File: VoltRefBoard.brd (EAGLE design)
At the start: 50 x 50 mm, 30 parts, among them J1 BANANA_CONN, J2 BANANA_CONN, J3 BANANA_CONN, J4 BANANA_CONN, J5 BANANA_CONN, U1 MAX6225ACSA+, U2 MAX6250ACSA+

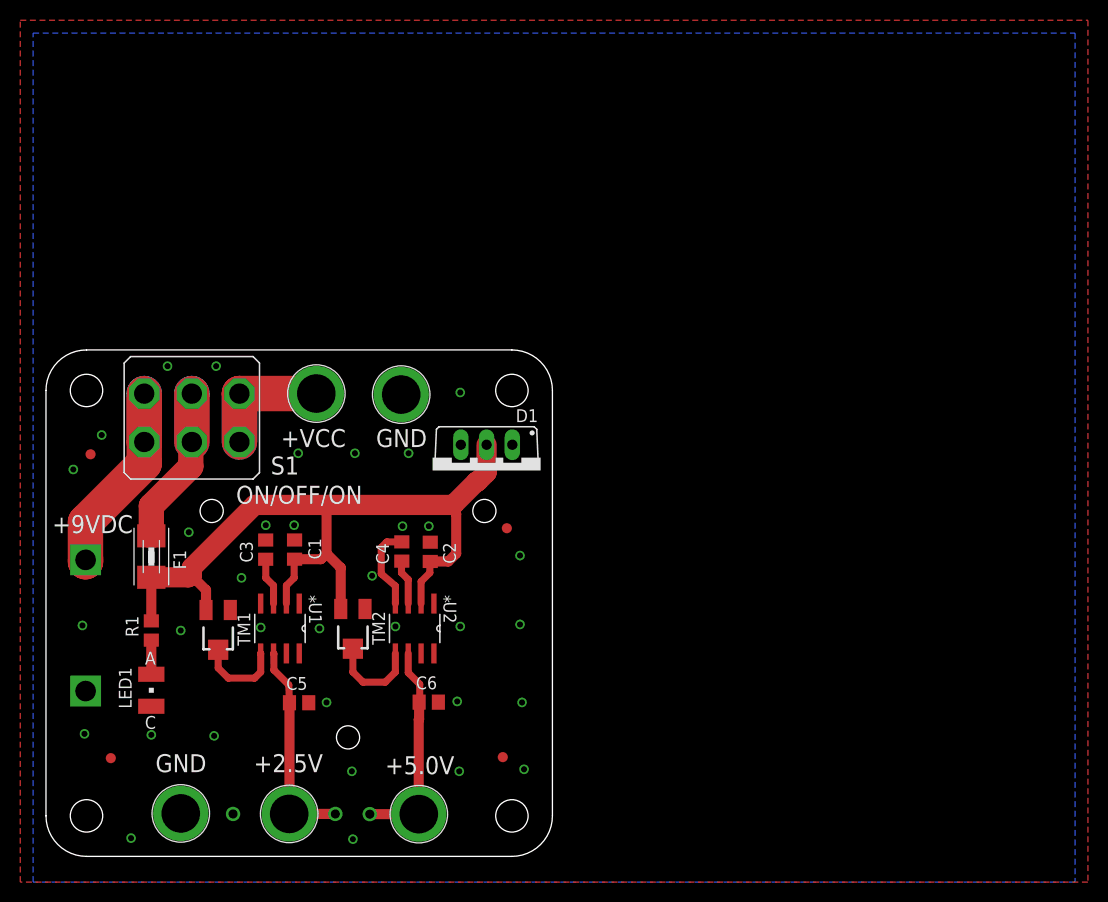
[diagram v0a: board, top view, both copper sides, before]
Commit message: adding latest updates
adding latest updates
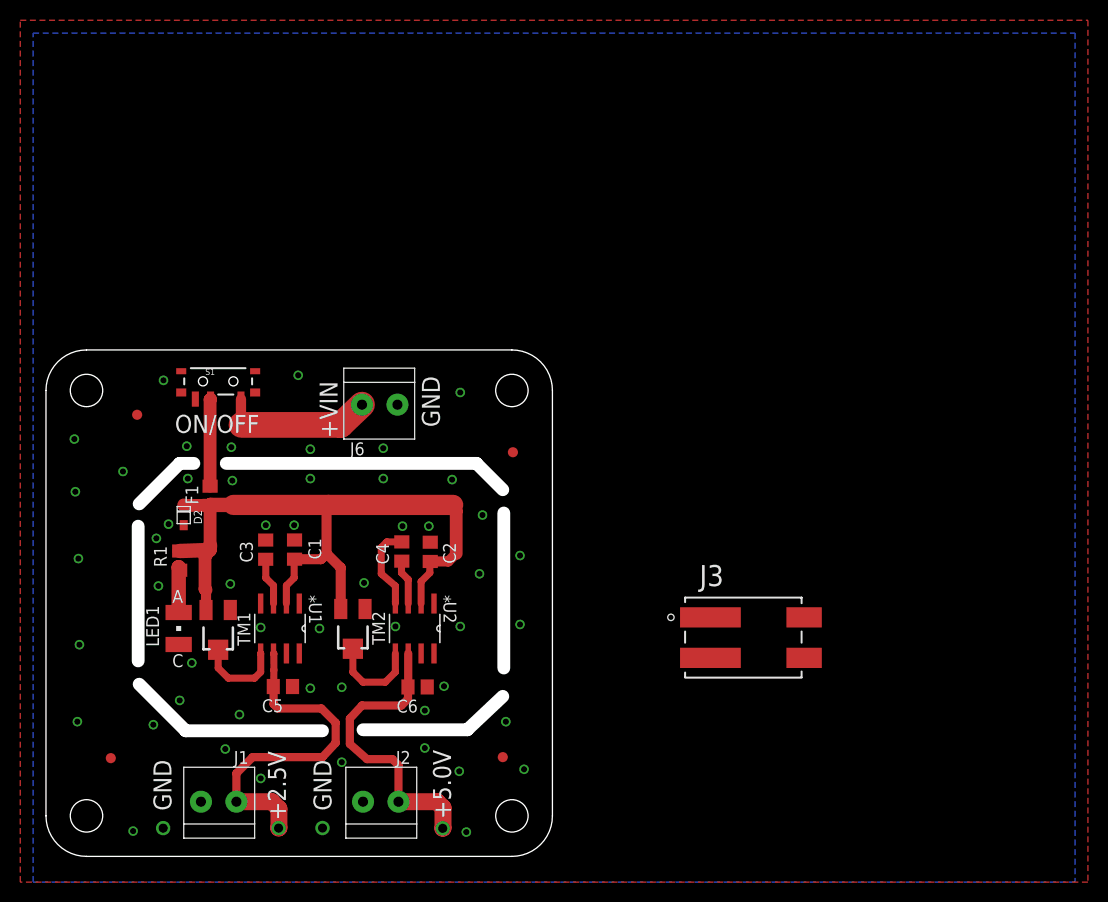
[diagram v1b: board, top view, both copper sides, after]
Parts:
- removed BAT1: +9V_BATTERY, BC9VPC_ShortenenSilkScreen:BC9VPC
- removed D1: MBR60H100CTG, diode:TO220ABS
- removed J4, J5: BANANA_CONN, SparkFun-Connectors:BANANA_CONN
- added D2: (no value), adafruit:SOD-323F
- added J6: 1X2-3.5MM, adafruit:1X2-3.5MM
- added TP4: TP_1MM_TH", TP_1MM_TH:TP_1MM_TH
- F1: value 1.1A -> PTC_0805_100MA; device adafruit:1812 -> rcl:R0805
- J1, J2: value BANANA_CONN -> 1X2-3.5MM; device SparkFun-Connectors:BANANA_CONN -> adafruit:1X2-3.5MM
- J3: value BANANA_CONN -> 2060-402; device SparkFun-Connectors:BANANA_CONN -> Wago-2060-402:WAGO_2060-402
- S1: value 5649A -> (none); device Switch_320-938_Corrected:320-938 -> SparkFun-Electromechanical:SWITCH-SPST-SMD-A
- moved J3 48.8 mm to (69.6, 21.6)
- moved J1 41.4 mm to (17.0, 5.40)
- moved J2 40.2 mm to (33.0, 5.40)
- moved F1 8.35 mm to (16.2, 35.6)
- moved U$3 7.52 mm to (46.1, 39.9)
- moved R1 7.45 mm to (13.2, 29.2)
- moved TP2 7.33 mm to (39.2, 2.77)
- moved TP3 7.04 mm to (11.6, 2.79)
- moved LED1 6.67 mm to (13.1, 22.5)
- moved U$4 6.03 mm to (9.00, 43.6)
- moved TP1 5.77 mm to (23.0, 2.79)
- moved S1 4.44 mm to (17.0, 46.9), turned to 0 degrees
- moved C5 2.26 mm to (23.4, 16.8)
- moved C6 1.86 mm to (36.7, 16.7)
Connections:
- removed net V_IN_B: BAT1.V+, S1.1, S1.4
- net +2.5V_REF: now also J1.1; no longer J3.P$1
- net +5.0V_REF: now also J2.1; no longer J4.P$1
- net GND: now also D2.A, J1.2, J2.2, J6.2, TP4.P$1; no longer BAT1.V-, D1.A1, D1.A2, J2.P$1, J5.P$1
- net V_IN_0: no longer S1.5
- net V_IN_1: now also D2.C; no longer D1.C
- net V_IN_A: now also J6.1; no longer J1.P$1, S1.6
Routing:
- net V_IN_B: track 24.0 -> 0.00 mm
- net +2.5V_REF: track 21.0 -> 34.6 mm
- net V_IN_0: track 20.5 -> 8.62 mm
- net V_IN_1: track 80.3 -> 72.0 mm
- net +5.0V_REF: track 21.2 -> 29.5 mm
- net V_IN_A: track 17.2 -> 15.3 mm
- net N$30: track 3.37 -> 4.79 mm
- net GND: vias 34 -> 52
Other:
- board text added: "+VIN"
- board text added: "ON/OFF"
- board text removed: "+9VDC"
- board text removed: "+VCC"
- board text removed: "-=BATTERY HOLDER THIS SIDE=-"
- board text removed: "ON/OFF/ON"

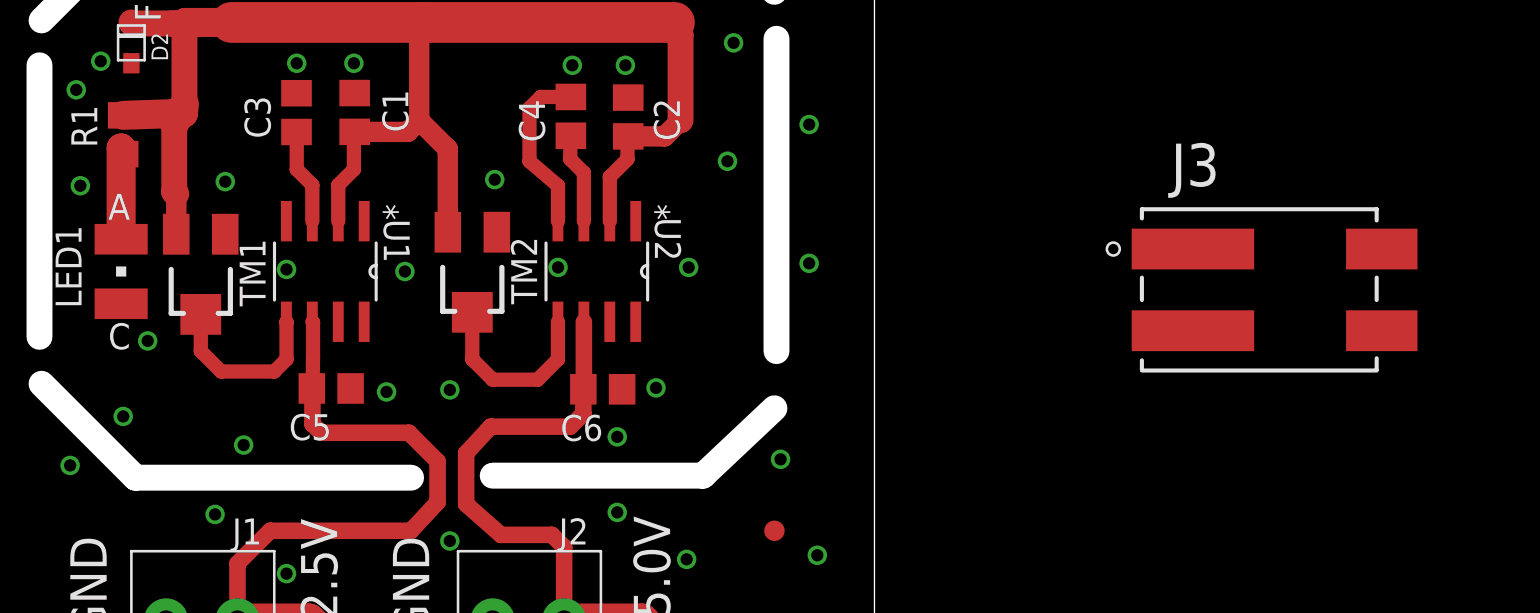
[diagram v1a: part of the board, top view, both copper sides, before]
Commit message: minor updates
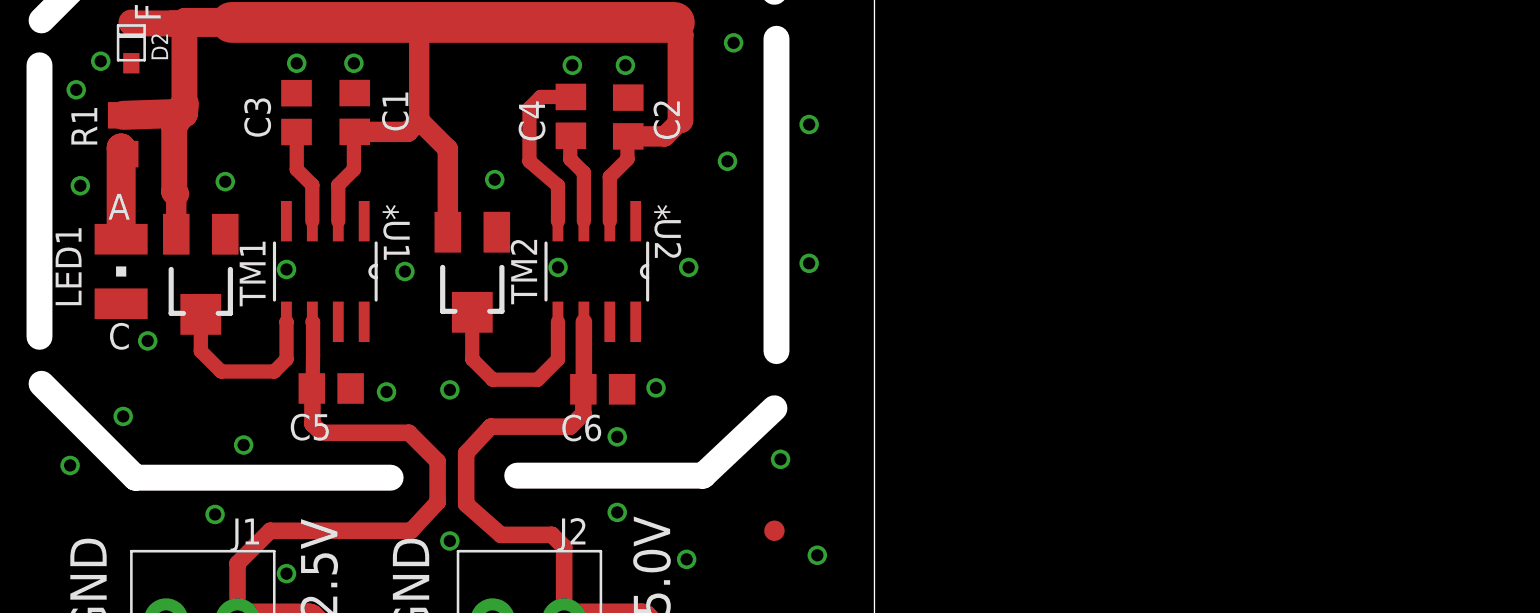
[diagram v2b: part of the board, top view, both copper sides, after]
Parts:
- removed J3: 2060-402, Wago-2060-402:WAGO_2060-402
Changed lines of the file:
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@@
 <text x="27.3" y="7.025" size="1.778" layer="25" rot="R270" align="center">GND</text>
 <text x="11.5" y="7.025" size="1.778" layer="25" rot="R270" align="center">GND</text>
-<wire x1="27.3" y1="12.4" x2="13.8" y2="12.4" width="1.27" layer="46"/>
+<wire x1="26.3" y1="12.4" x2="13.8" y2="12.4" width="1.27" layer="46"/>
 <wire x1="13.8" y1="12.4" x2="9.2" y2="17" width="1.27" layer="46"/>
-<wire x1="31.3" y1="12.5" x2="41.6" y2="12.5" width="1.27" layer="46"/>
+<wire x1="32.5" y1="12.5" x2="41.6" y2="12.5" width="1.27" layer="46"/>
 <wire x1="41.6" y1="12.5" x2="45.1" y2="15.8" width="1.27" layer="46"/>
 <wire x1="45.1" y1="36.2" x2="42.5" y2="38.8" width="1.27" layer="46"/>
@@
 <attribute name="VALUE" x="15.3" y="31.6" size="0.8128" layer="27" font="vector" rot="R90"/>
 </element>
-<element name="J3" library="Wago-2060-402" package="WAGO_2060-402" value="2060-402" x="69.6" y="21.6">
-<attribute name="MPN" value="2060-402/998-404" x="69.6" y="21.6" size="1.778" layer="27" display="off"/>
-<attribute name="OC_NEWARK" value="62T0379 " x="69.6" y="21.6" size="1.778" layer="27" display="off"/>
-<attribute name="PACKAGE" value="SMD-R/A" x="69.6" y="21.6" size="1.778" layer="27" display="off"/>
-<attribute name="SUPPLIER" value="WAGO" x="69.6" y="21.6" size="1.778" layer="27" display="off"/>
-<attribute name="OC_FARNELL" value="2102477 " x="69.6" y="21.6" size="1.778" layer="27" display="off"/>
-</element>
 </elements>
